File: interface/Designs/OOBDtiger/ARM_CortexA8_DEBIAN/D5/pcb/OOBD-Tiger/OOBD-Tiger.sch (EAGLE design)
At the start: 116 parts, among them IC1 ADM3053M, IC2 ADM3053M, IC4 DS3231, U1 SY6280, U10 MP1482DS, U2 SN65HVD230(SO8), U3 SY6280, U6 SN65HVD230(SO8)

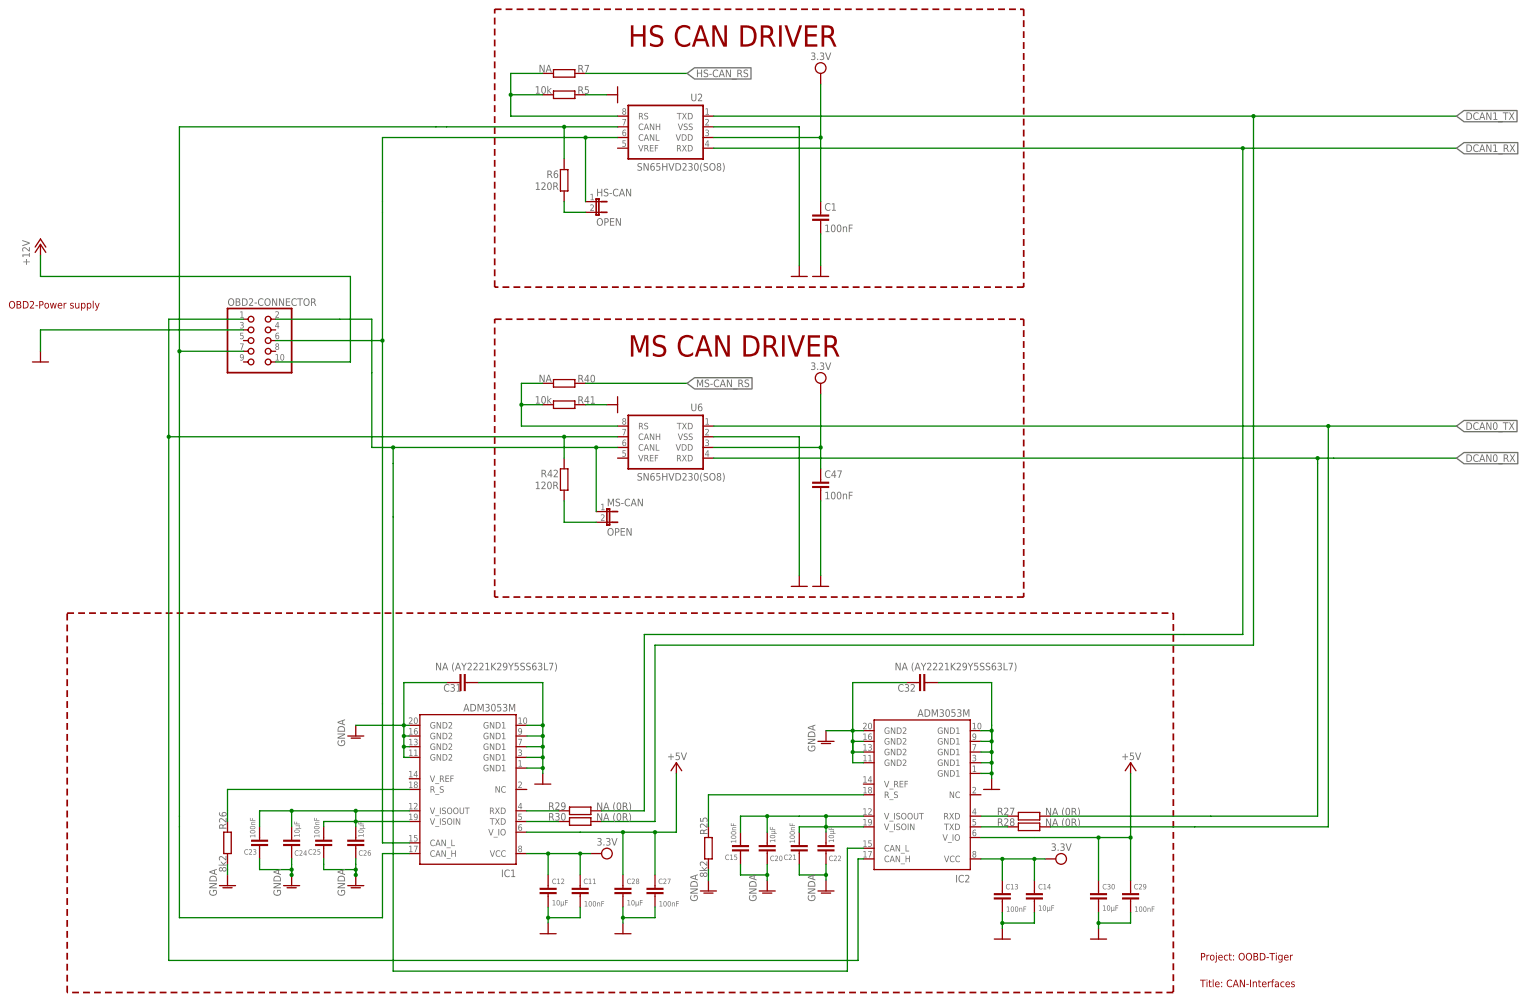
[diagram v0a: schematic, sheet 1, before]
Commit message: add latest modifications to OOBD schematics
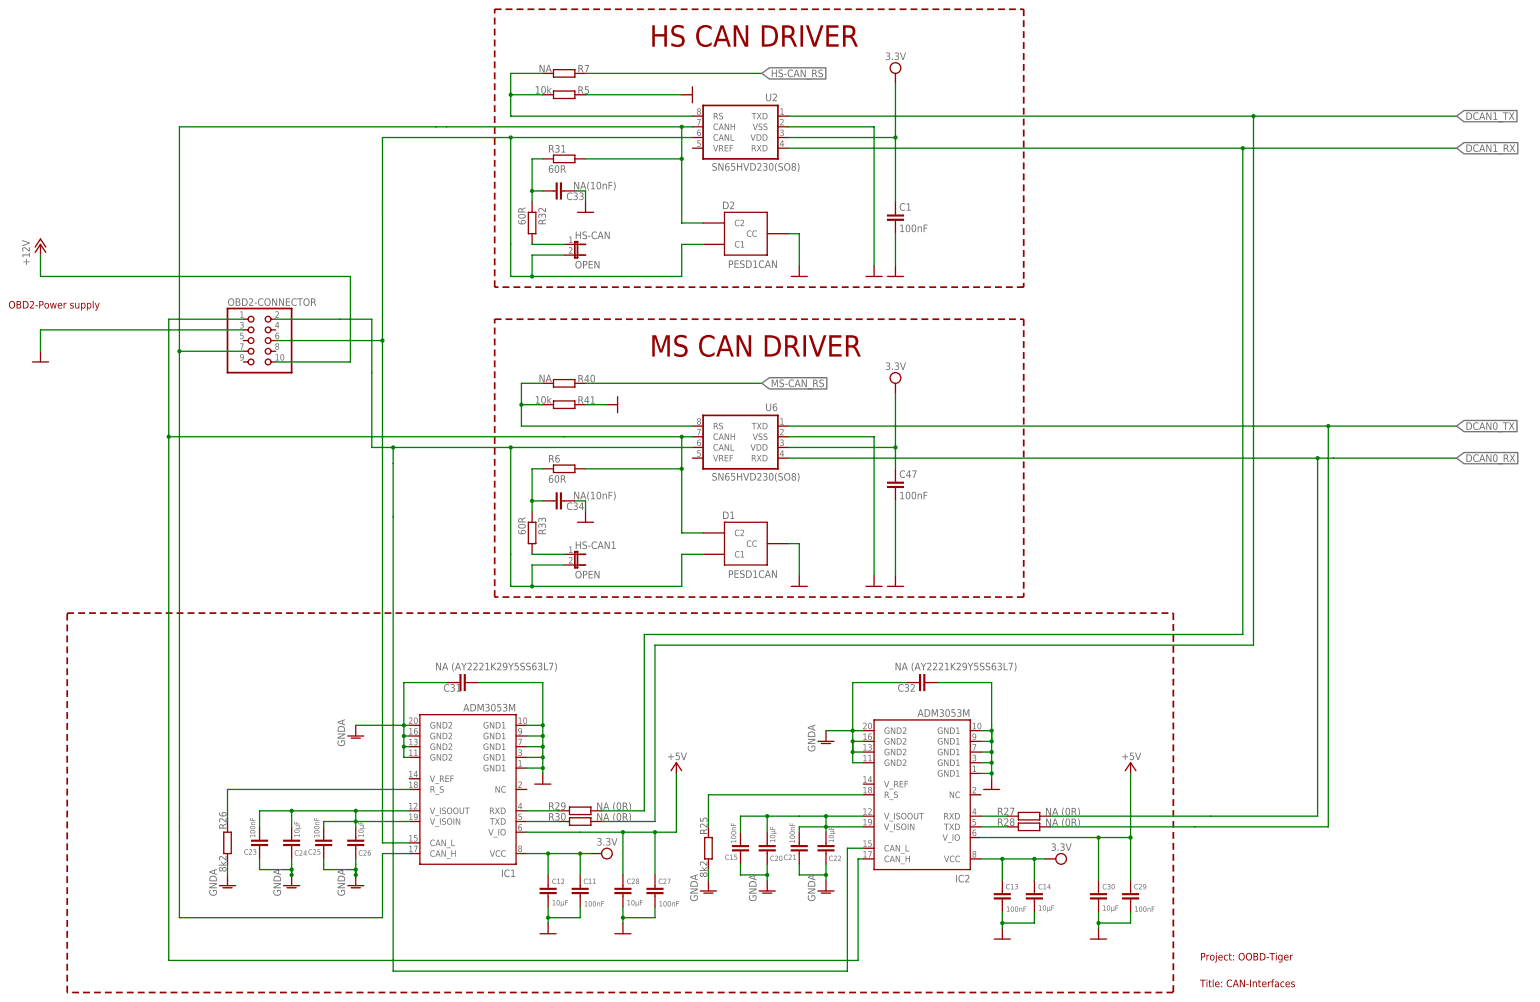
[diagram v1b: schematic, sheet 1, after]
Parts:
- removed MS-CAN: OPEN, SparkFun:JUMPER-2SMD-NO
- removed R42: 120R, rcl:R-EU_R0603
- added C33, C34: NA(10nF), resistor:C-EUC0603
- added D1, D2: PESD1CAN, Industrialberry:PESD1CAN
- added HS-CAN1: OPEN, SparkFun:JUMPER-2SMD-NO
- added R31, R32, R33: 60R, resistor:R-EU_R0603
- R6: value 120R -> 60R; device rcl:R-EU_R0603 -> resistor:R-EU_R0603
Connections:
- new net N$30: HS-CAN.1, R32.2
- new net N$32: HS-CAN1.1, R33.2
- net CAN0_H: now also D1.C2, R6.2; no longer R42.2
- net CAN0_L: now also D1.C1, HS-CAN1.2; no longer MS-CAN.1
- net CAN1_H: now also D2.C2, R31.2; no longer R6.2
- net CAN1_L: now also D2.C1, HS-CAN.2; no longer HS-CAN.1
- net GND: now also C33.2, C34.2, D1.CC, D2.CC
- net N$10: now also C34.1, R33.1, R6.1; no longer MS-CAN.2, R42.1
- net N$2: now also C33.1, R31.1, R32.1; no longer HS-CAN.2, R6.1
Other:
- moved on the sheet: C1, C47, HS-CAN, R6, U2, U6
